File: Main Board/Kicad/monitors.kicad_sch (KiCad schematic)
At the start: 3 parts, among them U5 INA3221, U6 INA3221, U7 INA3221

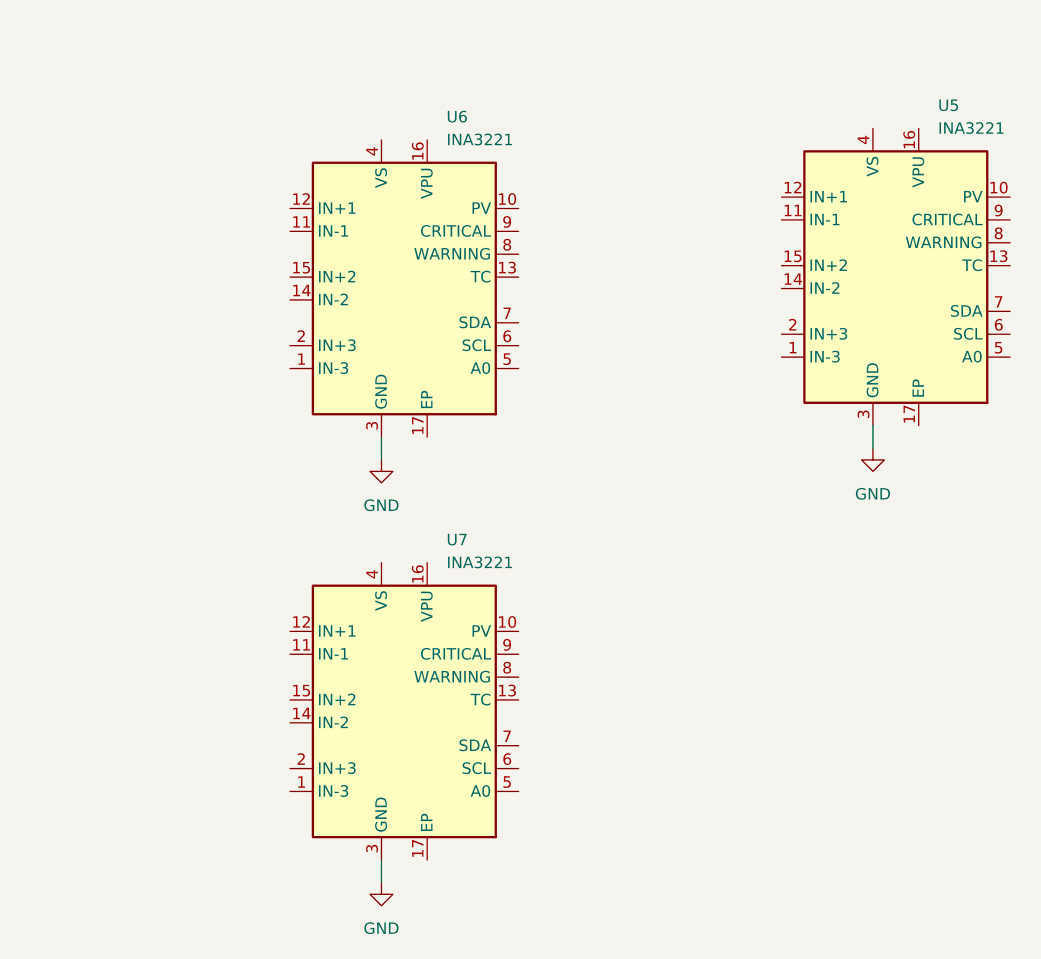
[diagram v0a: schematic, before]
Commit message: atualização pcb
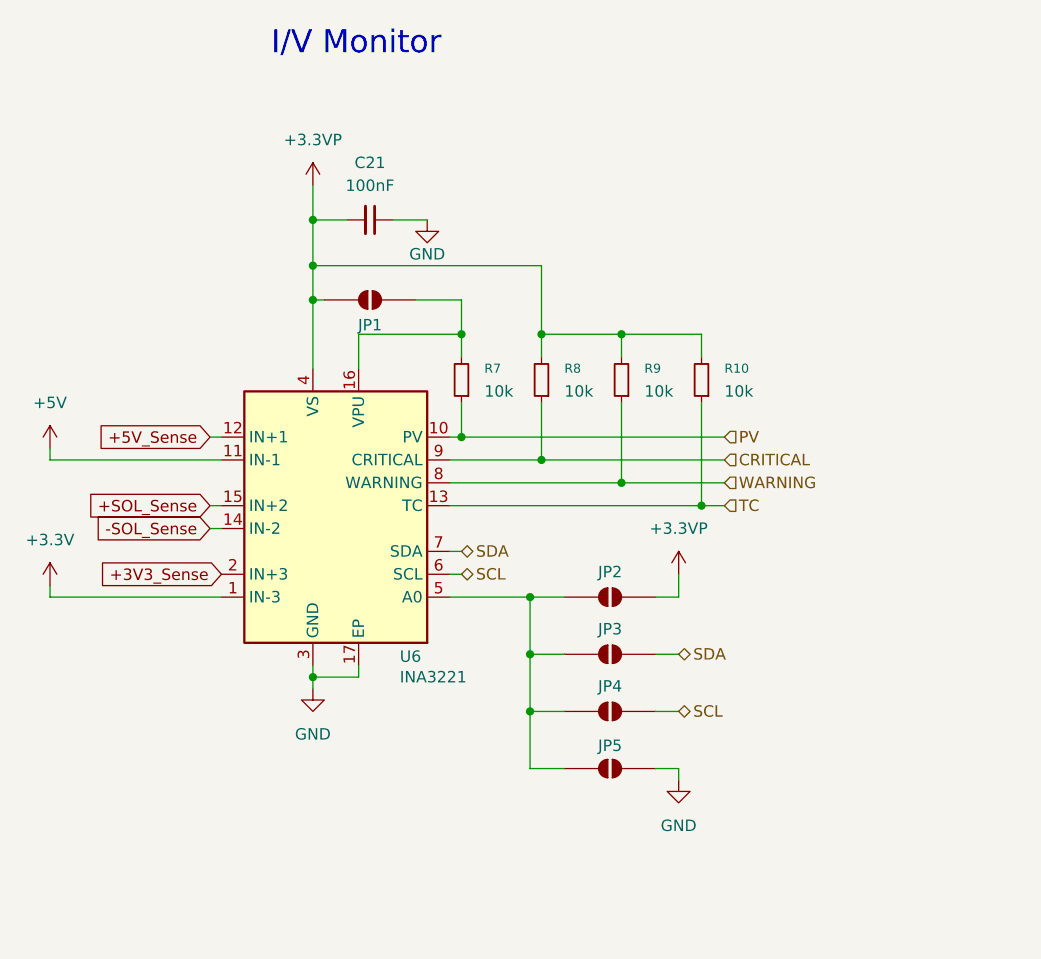
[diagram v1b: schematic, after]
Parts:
- removed U5, U7: INA3221, Package_DFN_QFN:Texas_RGV0016A_VQFN-16-1EP_4x4mm_P0.65mm_EP2.1x2.1mm, symbol Power_Management:INA3221
- added C21: 100nF, Capacitor_SMD:C_0402_1005Metric_Pad0.74x0.62mm_HandSolder, symbol Device:C_Small
- added JP1, JP2, JP3, JP4, JP5: SolderJumper_2_Open, Jumper:SolderJumper-2_P1.3mm_Open_RoundedPad1.0x1.5mm, symbol Jumper:SolderJumper_2_Open
- added R10, R7, R8, R9: 10k, Resistor_SMD:R_0402_1005Metric_Pad0.72x0.64mm_HandSolder, symbol Device:R_Small
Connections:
- net GND: now also U6.17 (EP), C21.1, JP5.2 (B)
- net +3.3V: now reaches U6.1 (IN-3)
- net PV: now reaches U6.10 (PV)
- net PV: now also R7.1
- net +5V: now reaches U6.11 (IN-1)
- net +5V_Sense: now reaches U6.12 (IN+1)
- net TC: now reaches U6.13 (TC)
- net TC: now also R10.1
- net -SOL_Sense: now reaches U6.14 (IN-2)
- net +SOL_Sense: now reaches U6.15 (IN+2)
- net at U6.16 (VPU): now also JP1.1 (A), R7.2
- net +3V3_Sense: now reaches U6.2 (IN+3)
- net +3.3VP: now reaches U6.4 (VS)
- net +3.3VP: now also C21.2, JP1.2 (B), JP2.2 (B), R10.2, R8.2, R9.2
- net at U6.5 (A0): now also JP2.1 (A), JP3.1 (A), JP4.1 (A), JP5.1 (A)
- net SCL: now reaches U6.6 (SCL)
- net SCL: now also JP4.2 (B)
- net SDA: now reaches U6.7 (SDA)
- net SDA: now also JP3.2 (B)
- net WARNING: now reaches U6.8 (WARNING)
- net WARNING: now also R9.1
- net CRITICAL: now reaches U6.9 (CRITICAL)
- net CRITICAL: now also R8.1
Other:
- note added: "I/V Monitor"
- moved on the sheet: U6
